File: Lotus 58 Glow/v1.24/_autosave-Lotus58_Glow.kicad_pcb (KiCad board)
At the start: 2 copper layers, 139.1 x 107.7 mm, 132 parts, among them J1 PJ-320A, J2 Conn_01x02, P1 OLED, SW1 Kailh hotswap MX socket, SW10 Kailh hotswap MX socket, SW11 Kailh hotswap MX socket, SW12 Kailh hotswap MX socket, SW13 Kailh hotswap MX socket, SW14 Kailh hotswap MX socket, SW15 Kailh hotswap MX socket, SW16 Kailh hotswap MX socket, SW17 Kailh hotswap MX socket, SW18 Kailh hotswap MX socket, SW19 Kailh hotswap MX socket, SW2 Kailh hotswap MX socket, SW20 Kailh hotswap MX socket, SW21 Kailh hotswap MX socket, SW22 Kailh hotswap MX socket, SW23 Kailh hotswap MX socket, SW24 Kailh hotswap MX socket, SW25 Kailh hotswap MX socket, SW26 Kailh hotswap MX socket, SW27 Kailh hotswap MX socket, SW28 Kailh hotswap MX socket, SW29 Kailh hotswap MX socket, SW3 Kailh hotswap MX socket, SW30 Rotary_Encoder_Switch, SW31 Rotary_Encoder_Switch, SW4 Kailh hotswap MX socket, SW5 Kailh hotswap MX socket, SW6 Kailh hotswap MX socket, SW7 Kailh hotswap MX socket, SW8 Kailh hotswap MX socket, SW9 Kailh hotswap MX socket, U1 ProMicro, U2 SRV05-4

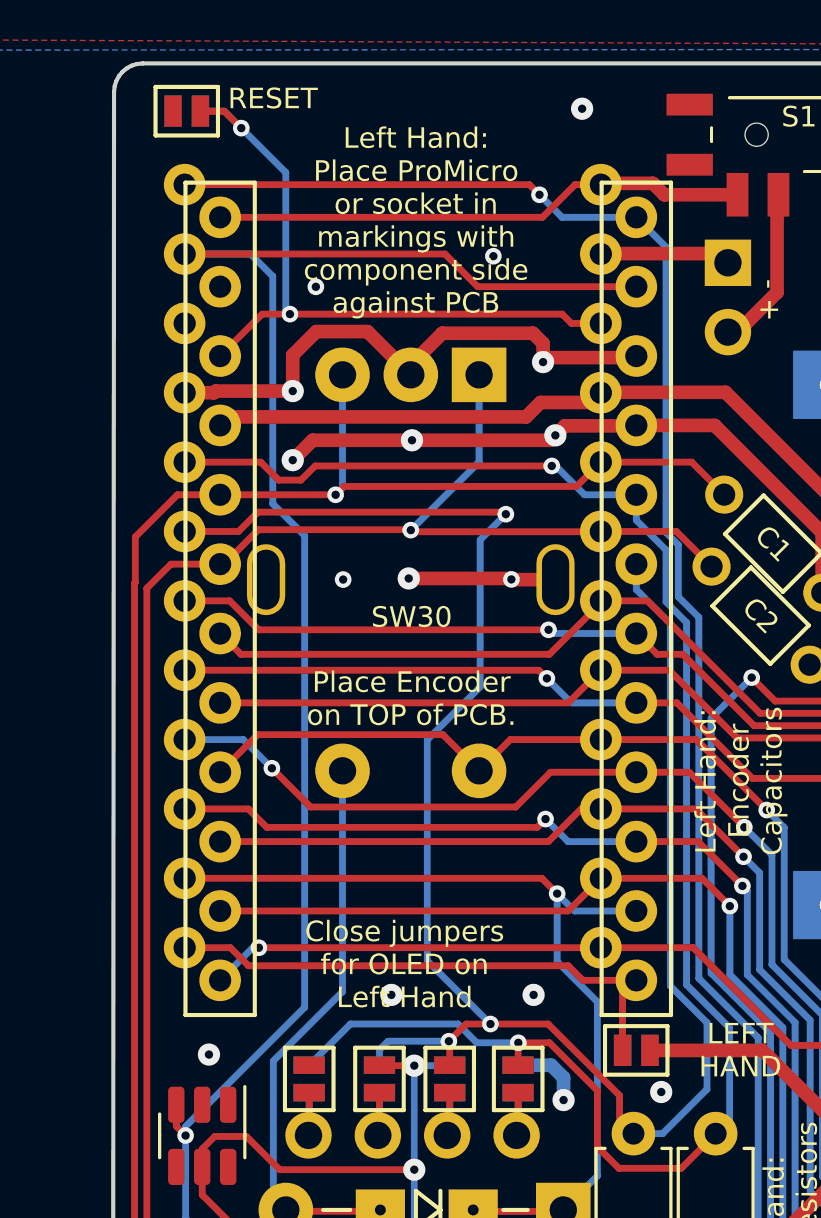
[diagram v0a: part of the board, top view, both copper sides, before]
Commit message: v1.24 tweaks
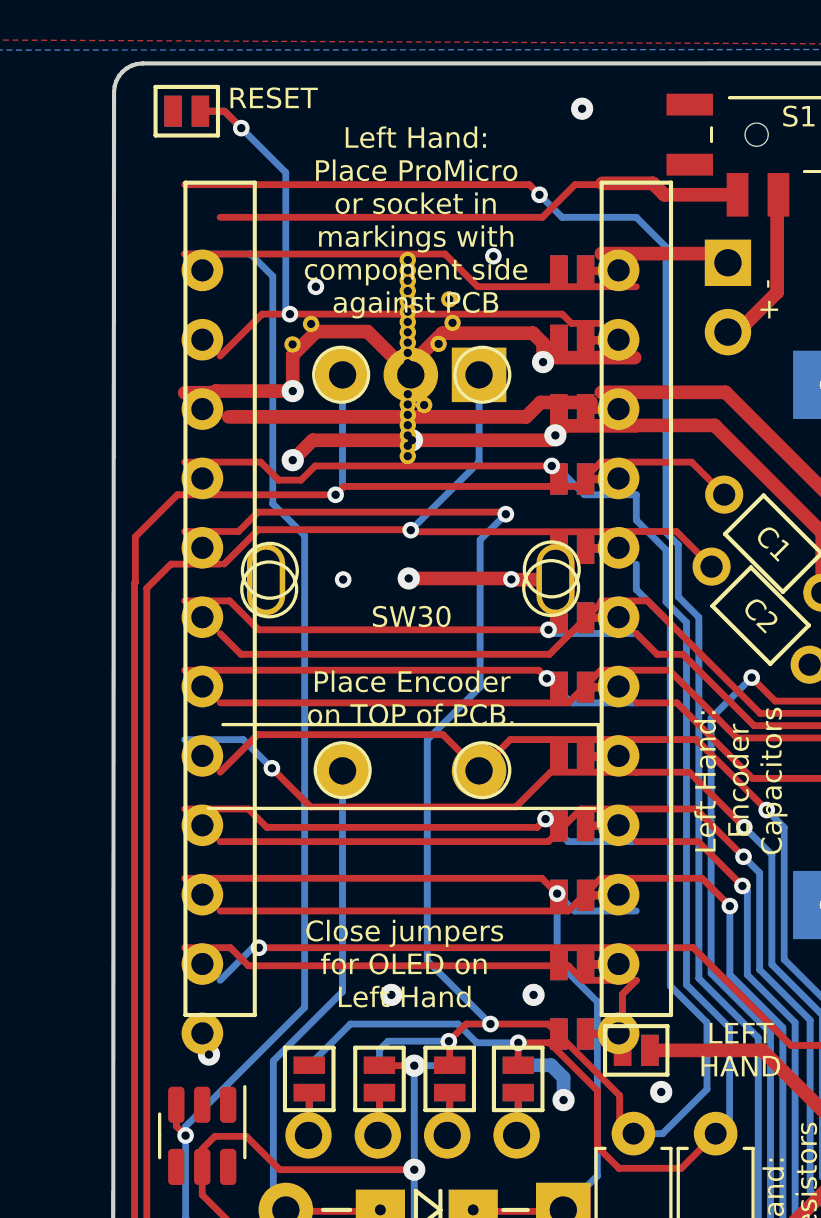
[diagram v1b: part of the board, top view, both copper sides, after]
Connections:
- U1 pad 1: LED -> (no net)
- U1 pad 10: row3 -> (no net)
- U1 pad 11: row4 -> (no net)
- U1 pad 12: Hand -> (no net)
- U1 pad 13: col3 -> (no net)
- U1 pad 14: col1 -> (no net)
- U1 pad 15: col2 -> (no net)
- U1 pad 16: col0 -> (no net)
- U1 pad 17: col4 -> (no net)
- U1 pad 18: col5 -> (no net)
- U1 pad 19: A -> (no net)
- U1 pad 20: B -> (no net)
- U1 pad 21: VCC -> (no net)
- U1 pad 22: RESET -> (no net)
- U1 pad 24: Battery -> (no net)
- U1 pad 3: GND -> (no net)
- U1 pad 4: GND -> (no net)
- U1 pad 5: SDA -> (no net)
- U1 pad 6: SCL -> (no net)
- U1 pad 7: row0 -> (no net)
- U1 pad 8: row1 -> (no net)
- U1 pad 9: row2 -> (no net)
